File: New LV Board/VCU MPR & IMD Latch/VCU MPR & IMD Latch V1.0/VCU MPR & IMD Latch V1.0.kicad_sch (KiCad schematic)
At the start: 15 parts, among them J1 691137710002, J2 B12B-PH-K-S, J4 691137710002, K1 ALF1PF12, K2 AHES4291, SW1 Test Reset IMD

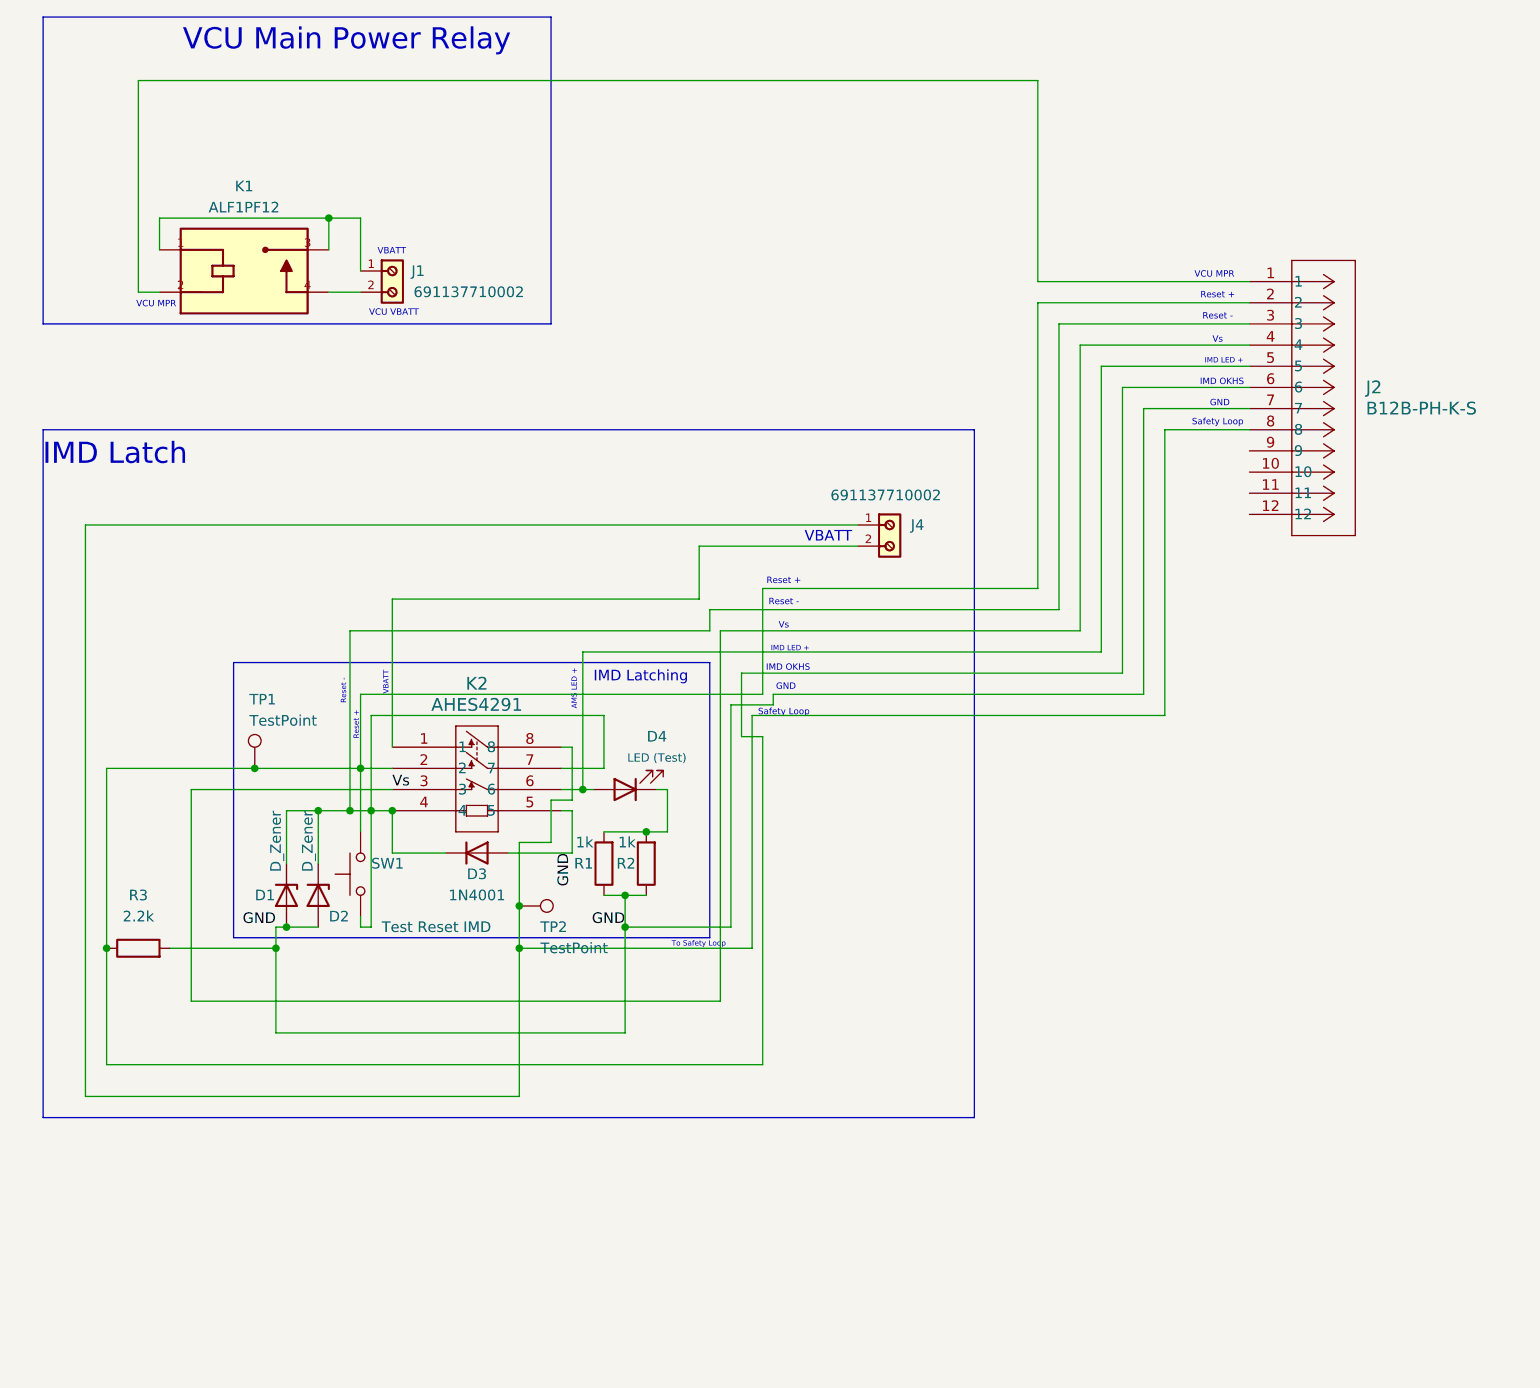
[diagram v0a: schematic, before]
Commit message: VCU MPR and IMP Latch
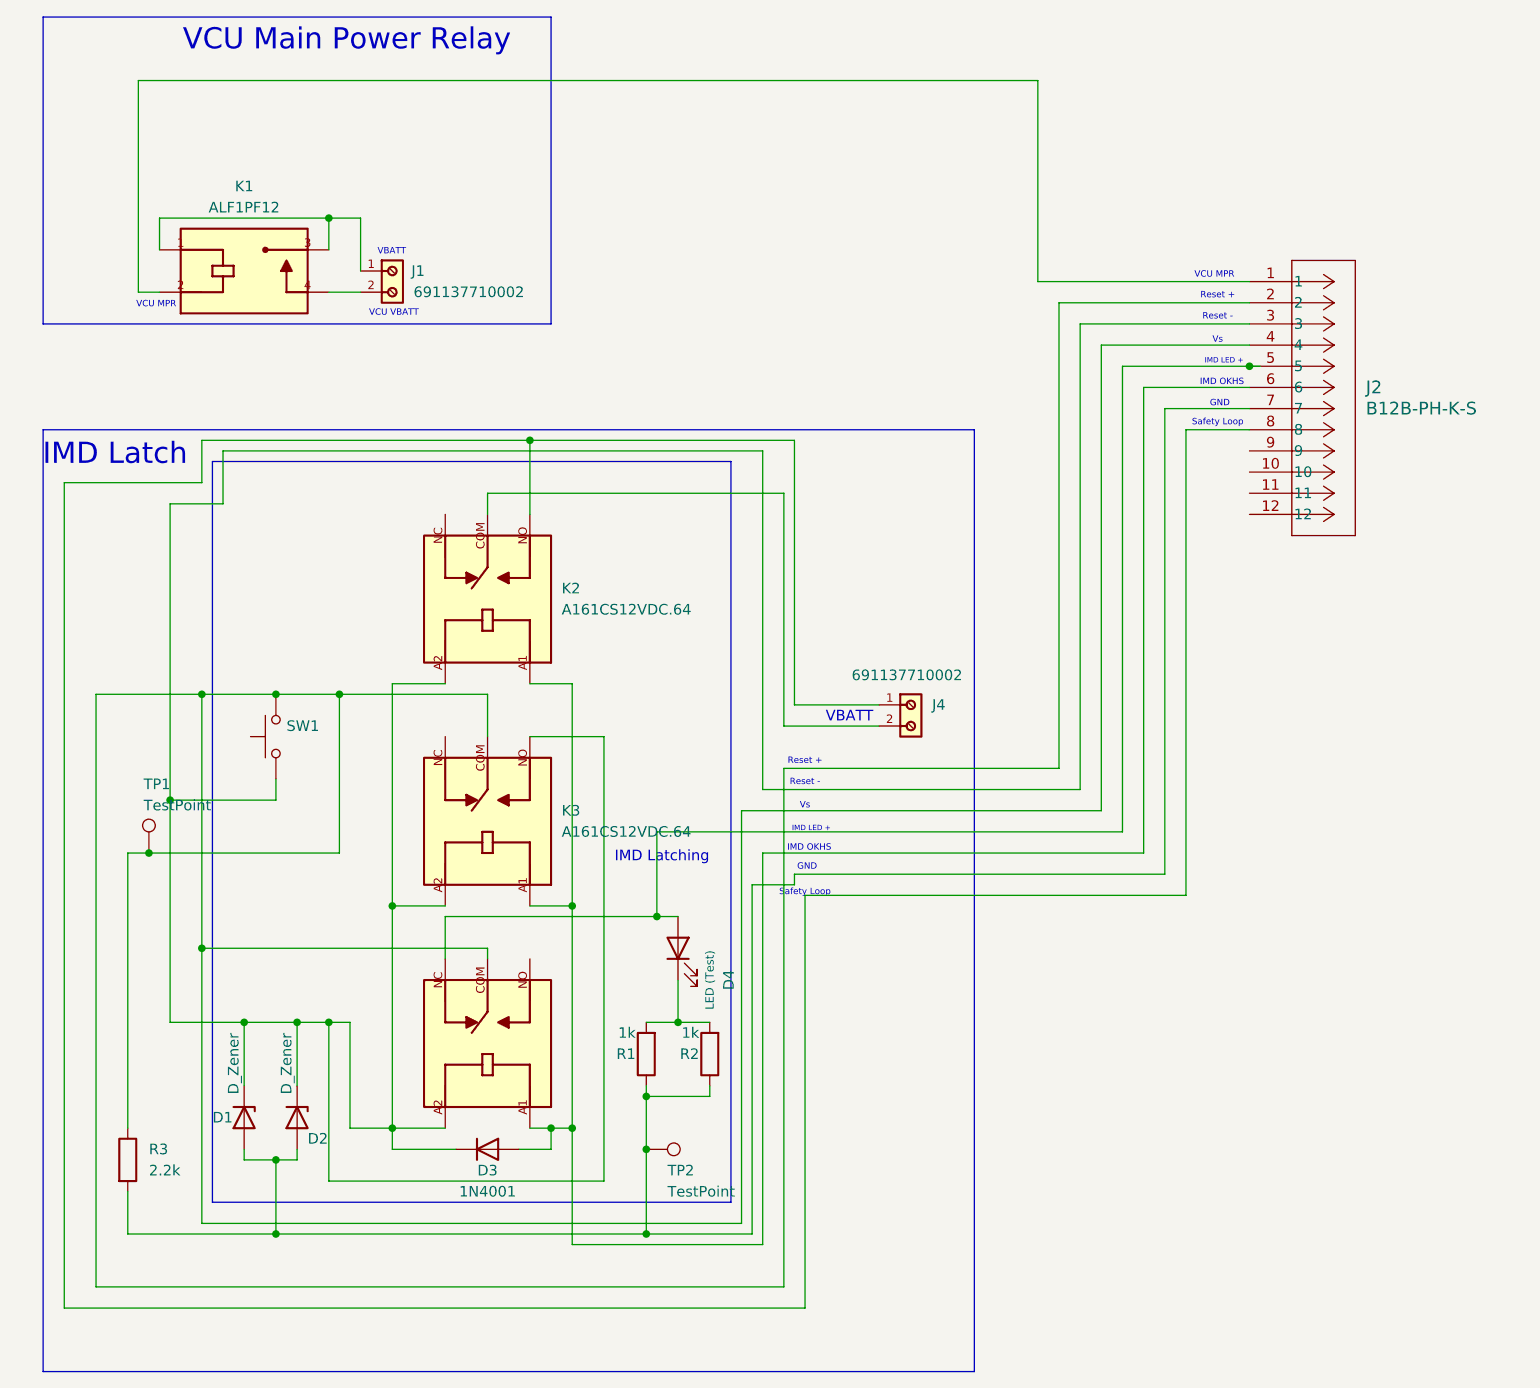
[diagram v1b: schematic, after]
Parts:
- removed K2: AHES4291, motorsports:AHES4_PAN, symbol Relay:AHES4291
- added K2, K3, K4: A161CS12VDC.64, A161CS12VDC.64:RELAY_A161CS12VDC.64, symbol New_Library:A161CS12VDC.64
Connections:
- net Vs is gone; now on an unnamed net: J2.4
- net at D4.2 (A), J2.5: now also K4.NC
- net at D1.1 (K), D2.1 (K), D3.1 (K)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: now also K2.A2, K3.A2, K3.NO, K4.A2
- net at J2.8, J4.1: now also K2.NO; no longer TP2.1
- net at J4.2: now also K2.COM
- net at J2.2, R3.1, SW1.2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: now also K3.COM, K4.COM; no longer J2.6
- net GND: no longer names the net of D1.2 (A), D2.2 (A), J2.7, R1.1, R2.1, R3.2
- net GND: now also TP2.1; no longer D3.2 (A)
- new net: D3.2 (A), J2.6, K2.A1, K3.A1, K4.A1
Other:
- note removed: "AMS LED +"
- note removed: "To Safety Loop"
- moved on the sheet: D1, D2, D3, D4, J4, R1, R2, R3, SW1, TP1, TP2

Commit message: Opening files forcing me to commit
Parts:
- K2, K3, K4: footprint A161CS12VDC.64:RELAY_A161CS12VDC.64 -> Library:RELAY_A161CS12VDC.64
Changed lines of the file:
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@@
 			)
 		)
-		(property "Footprint" "A161CS12VDC.64:RELAY_A161CS12VDC.64"
+		(property "Footprint" "Library:RELAY_A161CS12VDC.64"
 			(at 68.58 137.16 0)
 			(effects
@@
 			)
 		)
-		(property "Footprint" "A161CS12VDC.64:RELAY_A161CS12VDC.64"
+		(property "Footprint" "Library:RELAY_A161CS12VDC.64"
 			(at 68.58 110.49 0)
 			(effects
@@
 			)
 		)
-		(property "Footprint" "A161CS12VDC.64:RELAY_A161CS12VDC.64"
+		(property "Footprint" "Library:RELAY_A161CS12VDC.64"
 			(at 68.58 83.82 0)
 			(effects
